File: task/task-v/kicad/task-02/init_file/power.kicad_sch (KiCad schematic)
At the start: 95 parts, among them J1 VIN_CONN, J2 LOAD_CONN_1, J3 LOAD_CONN_2, J4 LOAD_CONN_3, J5 LOAD_CONN_4, Q1 FDMC86102, Q2 FDMC86102, U1 LM5116, U10 IC_3V3_4, U2 MIC5205-3.3YM5, U3 IC_LOAD_1, U4 IC_LOAD_2, U5 IC_LOAD_3, U6 IC_LOAD_4, U7 IC_3V3_1, U8 IC_3V3_2, U9 IC_3V3_3

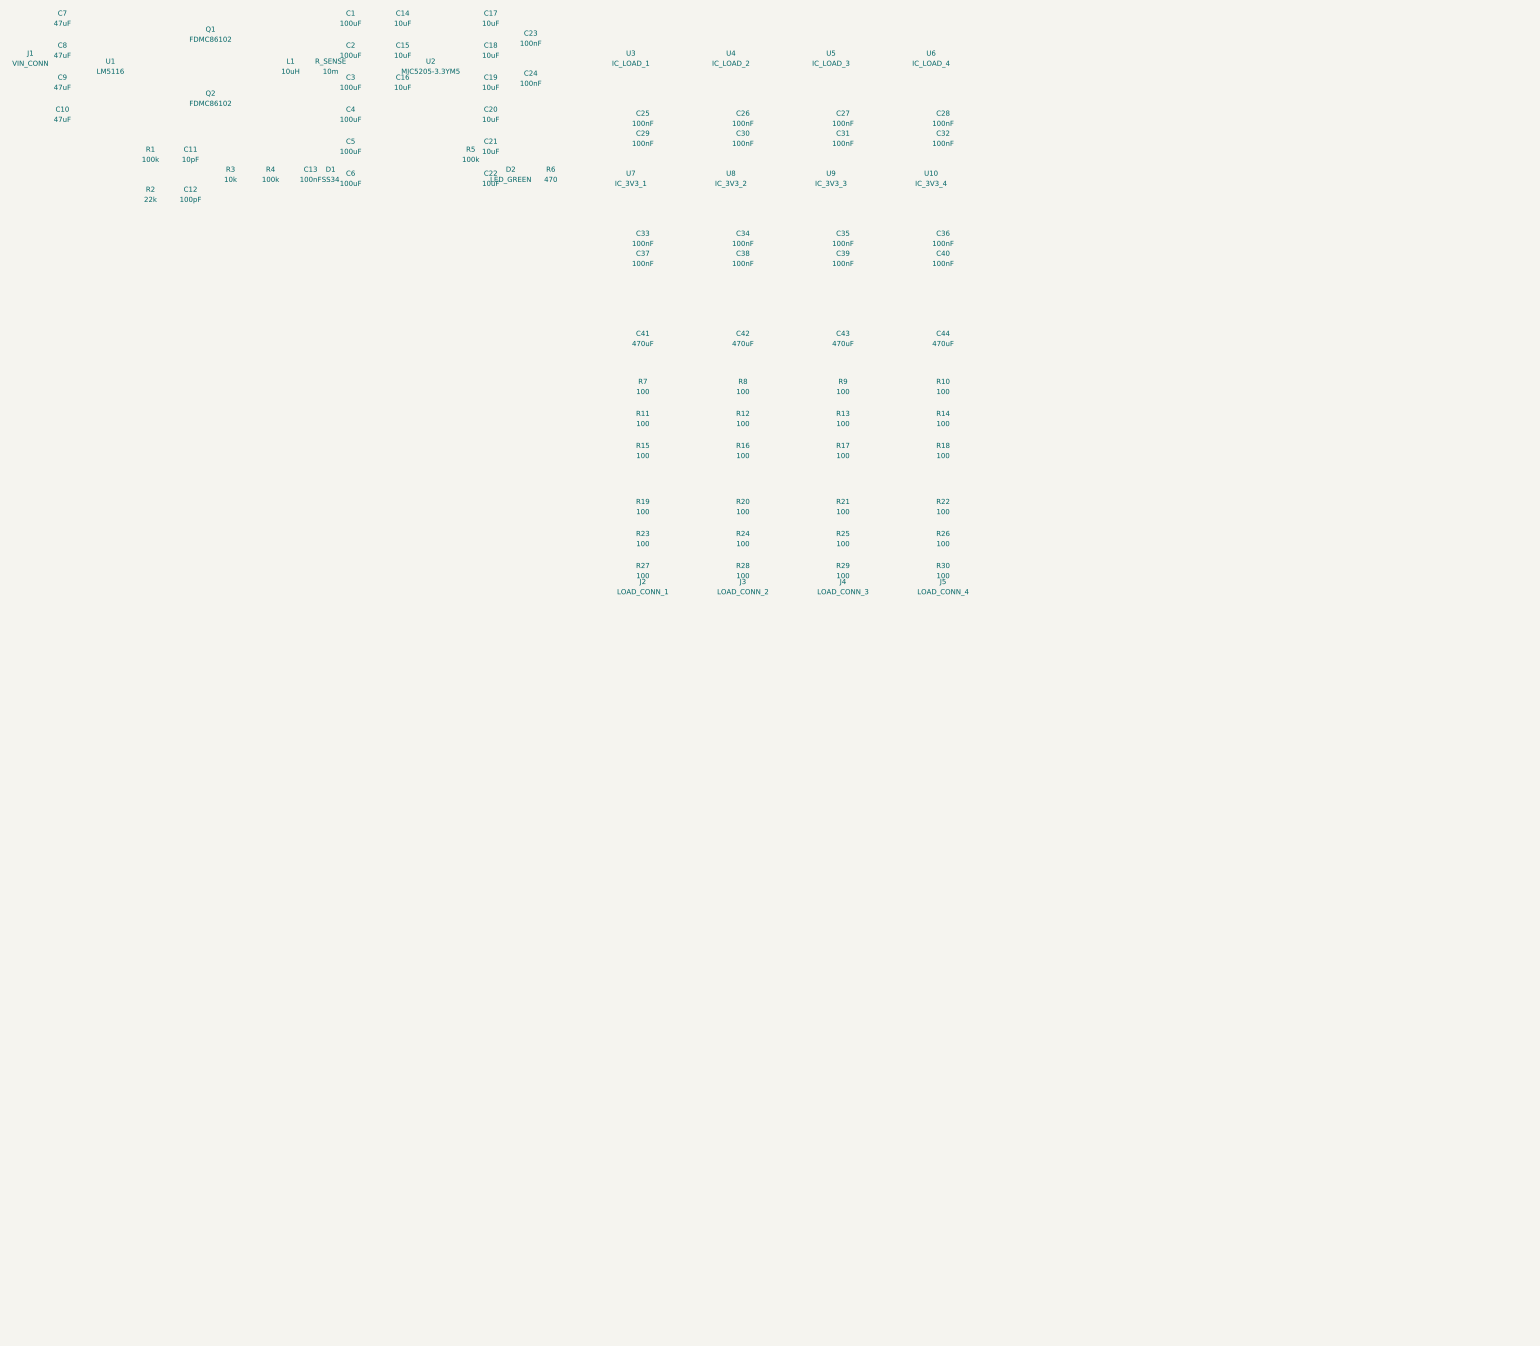
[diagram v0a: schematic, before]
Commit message: Repair KiCad 10.0.2 tasks and evaluators
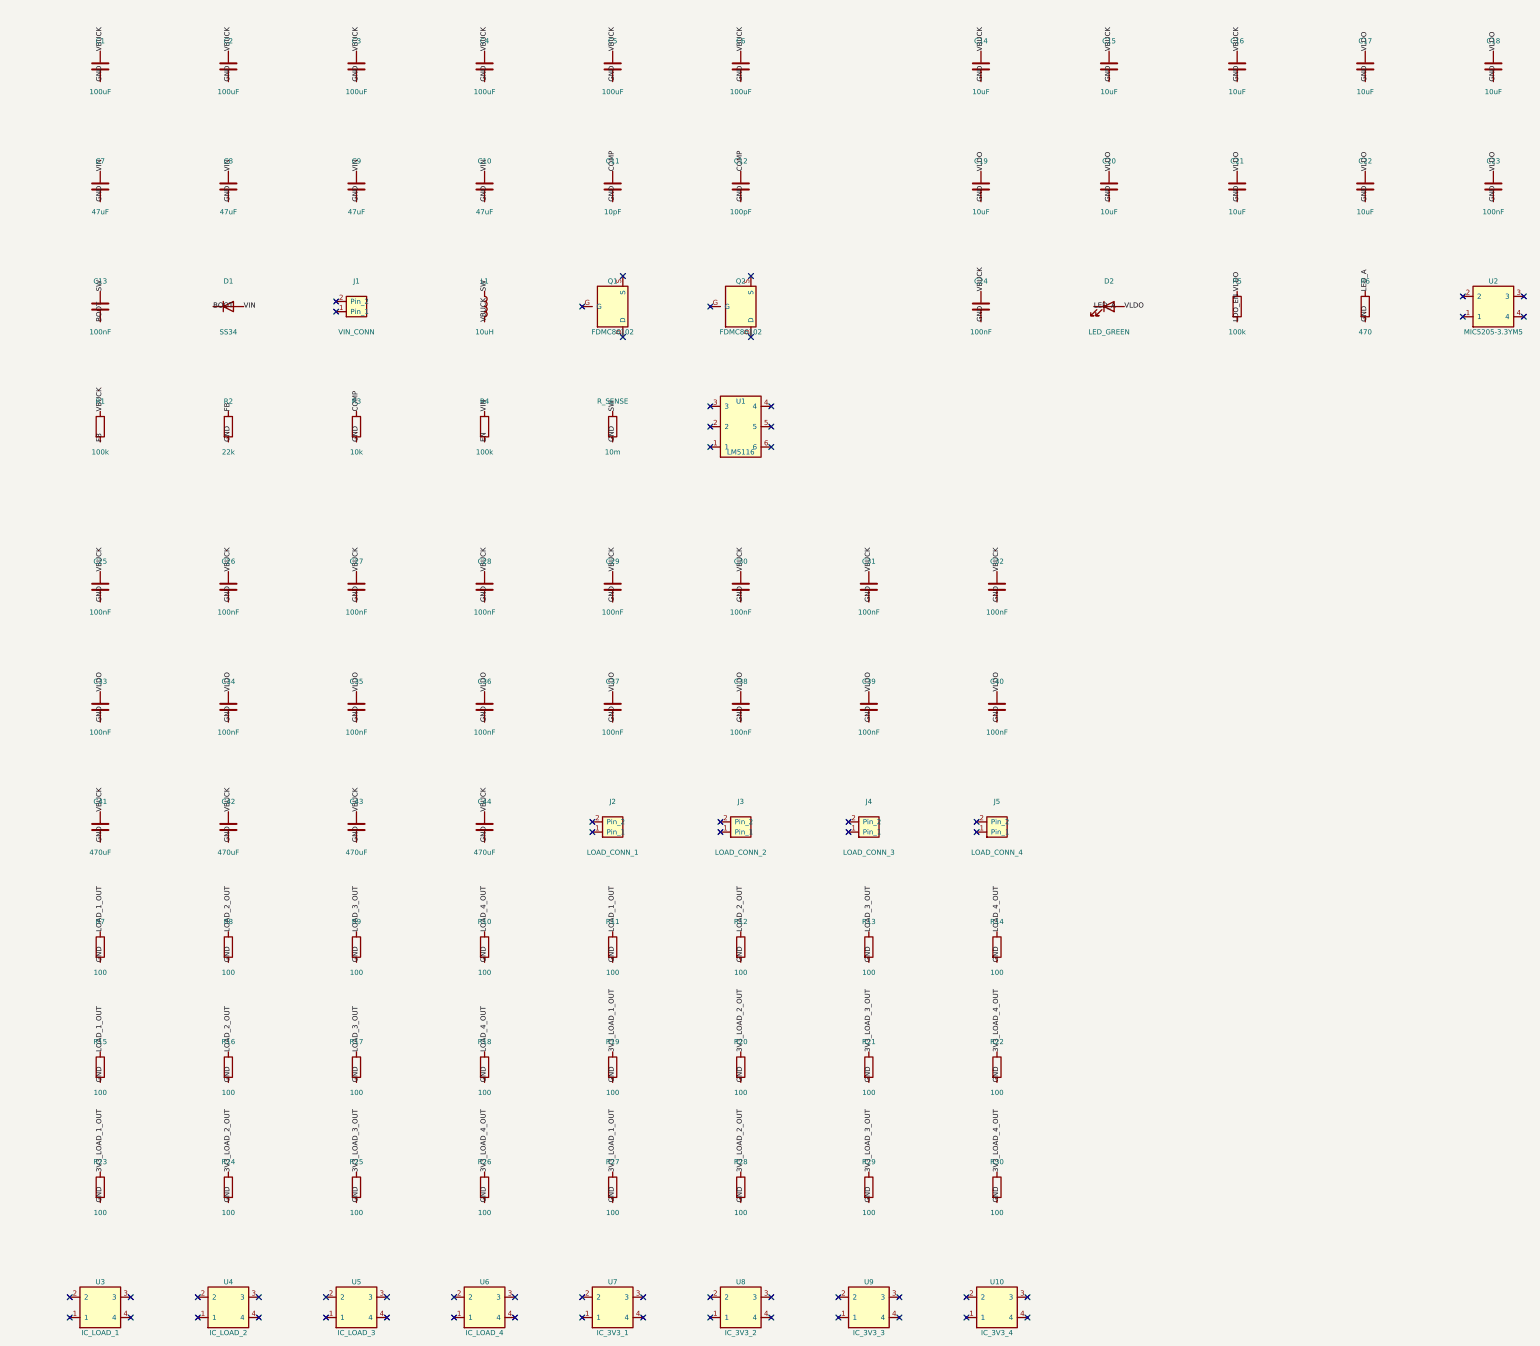
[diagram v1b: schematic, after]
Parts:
- removed D2: LED_GREEN, symbol Device:D
- removed J1: VIN_CONN, symbol Connector:Conn_01x02_Pin
- removed J2: LOAD_CONN_1, symbol Connector:Conn_01x02_Pin
- removed J3: LOAD_CONN_2, symbol Connector:Conn_01x02_Pin
- removed J4: LOAD_CONN_3, symbol Connector:Conn_01x02_Pin
- removed J5: LOAD_CONN_4, symbol Connector:Conn_01x02_Pin
- removed Q1, Q2: FDMC86102, symbol Device:Q_NMOS_GSD
- removed U1: LM5116, symbol Device:IC
- removed U10: IC_3V3_4, symbol Device:IC
- removed U2: MIC5205-3.3YM5, symbol Device:IC
- removed U3: IC_LOAD_1, symbol Device:IC
- removed U4: IC_LOAD_2, symbol Device:IC
- removed U5: IC_LOAD_3, symbol Device:IC
- removed U6: IC_LOAD_4, symbol Device:IC
- removed U7: IC_3V3_1, symbol Device:IC
- removed U8: IC_3V3_2, symbol Device:IC
- removed U9: IC_3V3_3, symbol Device:IC
- added D2: LED_GREEN, symbol Device:LED
- added J1: VIN_CONN, symbol Benchmark:Connector_02_Abstract
- added J2: LOAD_CONN_1, symbol Benchmark:Connector_02_Abstract
- added J3: LOAD_CONN_2, symbol Benchmark:Connector_02_Abstract
- added J4: LOAD_CONN_3, symbol Benchmark:Connector_02_Abstract
- added J5: LOAD_CONN_4, symbol Benchmark:Connector_02_Abstract
- added Q1, Q2: FDMC86102, symbol Benchmark:MOSFET_GSD_Abstract
- added U1: LM5116, symbol Benchmark:IC_06_Abstract
- added U10: IC_3V3_4, symbol Benchmark:IC_04_Abstract
- added U2: MIC5205-3.3YM5, symbol Benchmark:IC_04_Abstract
- added U3: IC_LOAD_1, symbol Benchmark:IC_04_Abstract
- added U4: IC_LOAD_2, symbol Benchmark:IC_04_Abstract
- added U5: IC_LOAD_3, symbol Benchmark:IC_04_Abstract
- added U6: IC_LOAD_4, symbol Benchmark:IC_04_Abstract
- added U7: IC_3V3_1, symbol Benchmark:IC_04_Abstract
- added U8: IC_3V3_2, symbol Benchmark:IC_04_Abstract
- added U9: IC_3V3_3, symbol Benchmark:IC_04_Abstract
- C1, C10, C11, C12, C13, C14, C15, C16, C17, C18, C19, C2, C20, C21, C22, C23, C24, C25, C26, C27, C28, C29, C3, C30, C31, C32, C33, C34, C35, C36, C37, C38, C39, C4, C40, C41, C42, C43, C44, C5, C6, C7, C8, C9, D1, L1, R1, R10, R11, R12, R13, R14, R15, R16, R17, R18, R19, R2, R20, R21, R22, R23, R24, R25, R26, R27, R28, R29, R3, R30, R4, R5, R6, R7, R8, R9, R_SENSE: ConnectivityScope (none) -> specified_by_source
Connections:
- new net 3V3_LOAD_1_OUT: R19.1, R23.1, R27.1
- new net 3V3_LOAD_2_OUT: R20.1, R24.1, R28.1
- new net 3V3_LOAD_3_OUT: R21.1, R25.1, R29.1
- new net 3V3_LOAD_4_OUT: R22.1, R26.1, R30.1
- new net BOOT: C13.2, D1.1 (K)
- new net COMP: C11.1, C12.1, R3.1
- new net EN: R4.2
- new net FB: R1.2, R2.1
- new net GND: C1.2, C10.2, C11.2, C12.2, C14.2, C15.2, C16.2, C17.2, C18.2, C19.2, C2.2, C20.2, C21.2, C22.2, C23.2, C24.2, C25.2, C26.2, C27.2, C28.2, C29.2, C3.2, C30.2, C31.2, C32.2, C33.2, C34.2, C35.2, C36.2, C37.2, C38.2, C39.2, C4.2, C40.2, C41.2, C42.2, C43.2, C44.2, C5.2, C6.2, C7.2, C8.2, C9.2, R10.2, R11.2, R12.2, R13.2, R14.2, R15.2, R16.2, R17.2, R18.2, R19.2, R2.2, R20.2, R21.2, R22.2, R23.2, R24.2, R25.2, R26.2, R27.2, R28.2, R29.2, R3.2, R30.2, R6.2, R7.2, R8.2, R9.2, R_SENSE.2
- new net LDO_EN: R5.2
- new net LED_A: D2.1 (K), R6.1
- new net LOAD_1_OUT: R11.1, R15.1, R7.1
- new net LOAD_2_OUT: R12.1, R16.1, R8.1
- new net LOAD_3_OUT: R13.1, R17.1, R9.1
- new net LOAD_4_OUT: R10.1, R14.1, R18.1
- new net SW: C13.1, L1.1, R_SENSE.1
- new net VBUCK: C1.1, C14.1, C15.1, C16.1, C2.1, C24.1, C25.1, C26.1, C27.1, C28.1, C29.1, C3.1, C30.1, C31.1, C32.1, C4.1, C41.1, C42.1, C43.1, C44.1, C5.1, C6.1, L1.2, R1.1
- new net VIN: C10.1, C7.1, C8.1, C9.1, D1.2 (A), R4.1
- new net VLDO: C17.1, C18.1, C19.1, C20.1, C21.1, C22.1, C23.1, C33.1, C34.1, C35.1, C36.1, C37.1, C38.1, C39.1, C40.1, D2.2 (A), R5.1
- no-connect marks 0 -> 58
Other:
- company: SCH01 Benchmark -> EngiWorld
- title: Power Supply - Flat Schematic -> Abstract Power Connectivity Fixture
